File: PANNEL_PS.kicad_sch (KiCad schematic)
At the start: 19 parts, among them IC30 TPS25940ARVCR, IC31 INA226AIDGSR

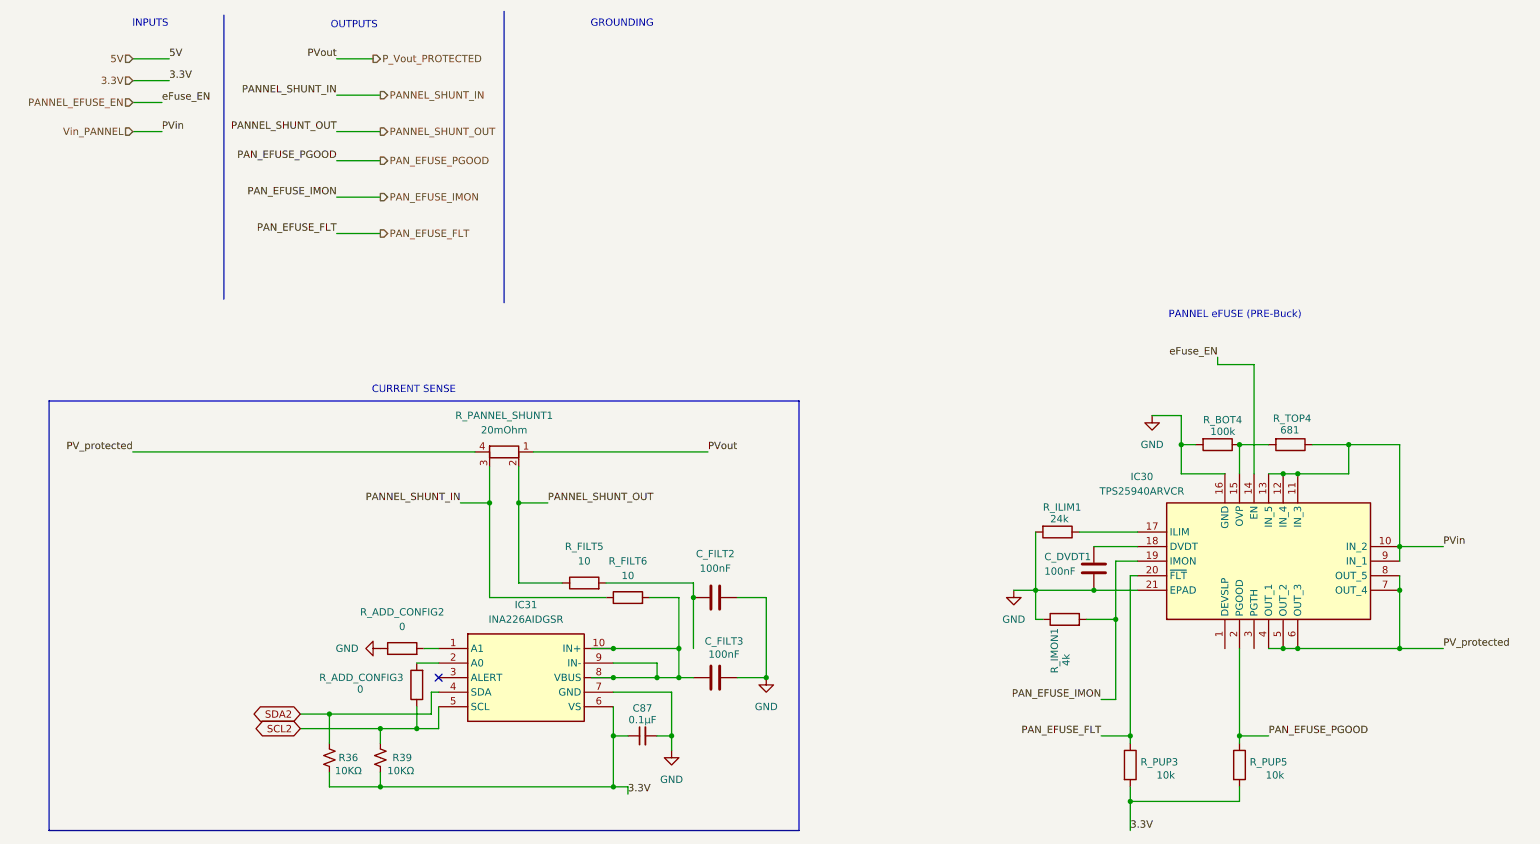
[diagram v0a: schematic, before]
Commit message: lastest
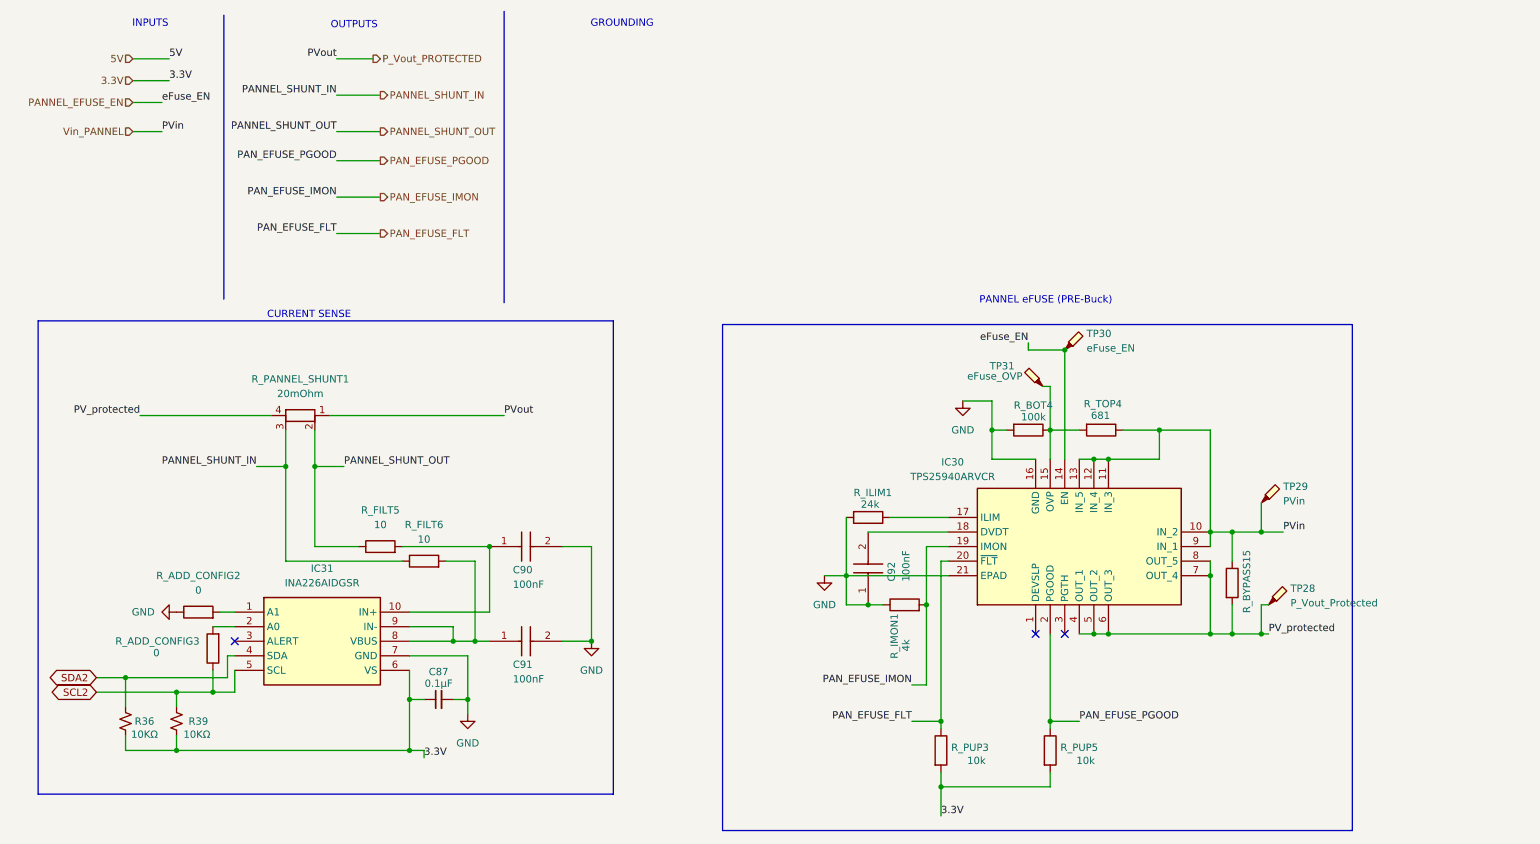
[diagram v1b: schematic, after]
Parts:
- removed C_DVDT1, C_FILT2, C_FILT3: 100nF, symbol Device:C
- added C90, C91, C92: 100nF, Capacitor_SMD:C_0603_1608Metric, symbol PULSE_Library:C0603X6S0J104M030BC
- added R_BYPASS15: 0, Resistor_SMD:R_0603_1608Metric, symbol Device:R
- added TP28: P_Vout_Protected, TestPoint:TestPoint_Pad_D2.0mm, symbol Connector:TestPoint_Probe
- added TP29: PVin, TestPoint:TestPoint_Pad_D2.0mm, symbol Connector:TestPoint_Probe
- added TP30: eFuse_EN, TestPoint:TestPoint_Pad_D2.0mm, symbol Connector:TestPoint_Probe
- added TP31: eFuse_OVP, TestPoint:TestPoint_Pad_D2.0mm, symbol Connector:TestPoint_Probe
- C87: footprint C0603 -> PULSE_Library:C0603
- IC31: footprint SOP50P490X110-10N -> PULSE_Library:SOP50P490X110-10N
- R36, R39: footprint RESC1608X55N -> PULSE_Library:RESC1608X55N
- R_ADD_CONFIG2, R_ADD_CONFIG3, R_BOT4, R_FILT5, R_FILT6, R_ILIM1, R_IMON1, R_PUP3, R_PUP5, R_TOP4: footprint (none) -> Resistor_SMD:R_0603_1608Metric
- R_PANNEL_SHUNT1: footprint (none) -> Resistor_SMD:R_Shunt_Vishay_WSKW0612
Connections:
- net GND: now also C90.2, C91.2, C92.1
- net PANNEL_EFUSE_EN: now also TP30.1
- net PV_protected: now also R_BYPASS15.2, TP28.1
- net Vin_PANNEL: now also R_BYPASS15.1, TP29.1
- net at IC31.8 (VBUS), IC31.9 (IN-), R_FILT6.2: now also C91.1; no longer IC31.10 (IN+)
- net at R_FILT5.2: now also IC31.10 (IN+), C90.1
- net at IC30.15 (OVP), R_BOT4.1, R_TOP4.2: now also TP31.1
- net at IC30.18 (DVDT): now also C92.2
- no-connect marks 1 -> 3
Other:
- moved on the sheet: C87, IC30, IC31, R36, R39, R_ADD_CONFIG2, R_ADD_CONFIG3, R_BOT4, R_FILT5, R_FILT6, R_ILIM1, R_IMON1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
